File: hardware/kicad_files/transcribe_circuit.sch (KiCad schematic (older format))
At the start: 23 parts, among them J1 europower, J2 RS232_SERIAL, J3 RS232_DSUB, J4 MIDI_IN_TRS, J5 MIDI_IN_DIN, J6 MIDI_OUT_TRS, J7 MIDI_OUT_DIN, U1 ProMicro, U2 MAX232, U3 6N137, U4 4069, U5 usbHostMini, U6 L78L33_TO92

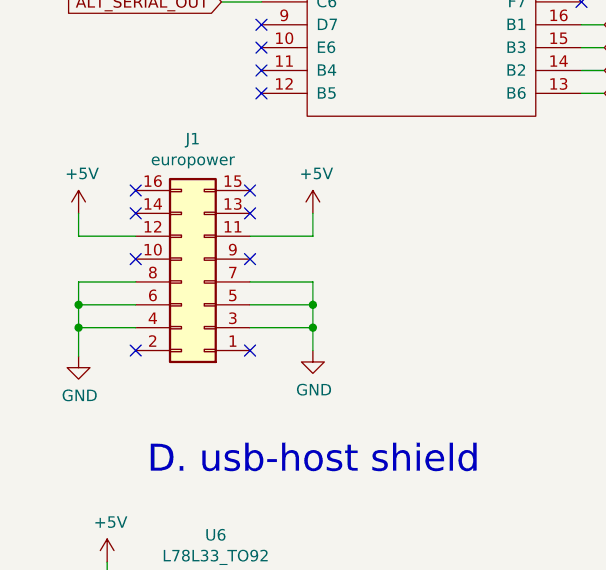
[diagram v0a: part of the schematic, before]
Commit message: small pcb fixes
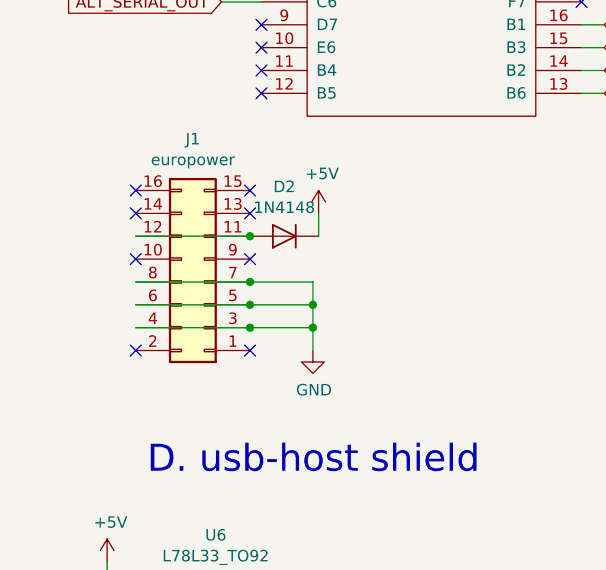
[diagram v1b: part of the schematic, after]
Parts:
- added D2: 1N4148, Diode_THT:D_T-1_P5.08mm_Horizontal, symbol Device:D
- C1: footprint Capacitor_THT:CP_Radial_D6.3mm_P2.50mm -> Capacitor_THT:CP_Radial_D5.0mm_P2.50mm
- C2, C3, C4, C5: footprint Capacitor_THT:C_Disc_D3.0mm_W1.6mm_P2.50mm -> Capacitor_THT:C_Disc_D4.3mm_W1.9mm_P5.00mm
- D1: footprint Diode_THT:D_A-405_P7.62mm_Horizontal -> Diode_THT:D_T-1_P5.08mm_Horizontal
- J1: footprint Connector_PinHeader_2.54mm:PinHeader_2x08_P2.54mm_Vertical -> lib_fp:PinHeader_2x08_P2.54_Euro
- J2, J4, J6: footprint Connector_Audio:Tayda_3.5mm_stereo_TRS_jack_A-853 -> lib_fp:Tayda_3.5mm_stereo_TRS_jack_A-853
- J5, J7: footprint Connector_DIN:Tayda5pinMidi-A1010 -> lib_fp:Tayda5pinMidi-A1010
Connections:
- net +5V: now also D2.1 (K); no longer J1.11 (Pin_11), J1.12 (Pin_12)
- new net: D2.2 (A), J1.11 (Pin_11), J1.12 (Pin_12)
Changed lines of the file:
@@
 F 0 "D1" V 8529 2129 50  0000 L CNN
 F 1 "1N4148" H 8475 1950 50  0000 L CNN
-F 2 "Diode_THT:D_A-405_P7.62mm_Horizontal" H 8575 2050 50  0001 C CNN
+F 2 "Diode_THT:D_T-1_P5.08mm_Horizontal" H 8575 2050 50  0001 C CNN
 F 3 "~" H 8575 2050 50  0001 C CNN
 	1    8575 2050
@@
 F 0 "J4" H 7632 3700 50  0000 C CNN
 F 1 "MIDI_IN_TRS" H 7632 3609 50  0000 C CNN
-F 2 "Connector_Audio:Tayda_3.5mm_stereo_TRS_jack_A-853" H 7650 3375 50  0001 C CNN
+F 2 "lib_fp:Tayda_3.5mm_stereo_TRS_jack_A-853" H 7650 3375 50  0001 C CNN
 F 3 "~" H 7650 3375 50  0001 C CNN
 	1    7650 3375
@@
 F 0 "J6" H 7707 6025 50  0000 C CNN
 F 1 "MIDI_OUT_TRS" H 7707 5934 50  0000 C CNN
-F 2 "Connector_Audio:Tayda_3.5mm_stereo_TRS_jack_A-853" H 7725 5700 50  0001 C CNN
+F 2 "lib_fp:Tayda_3.5mm_stereo_TRS_jack_A-853" H 7725 5700 50  0001 C CNN
 F 3 "~" H 7725 5700 50  0001 C CNN
 	1    7725 5700
@@
 F 0 "C2" H 4265 2971 50  0000 L CNN
 F 1 "0.1u" H 4265 2880 50  0000 L CNN
-F 2 "Capacitor_THT:C_Disc_D3.0mm_W1.6mm_P2.50mm" H 4188 2775 50  0001 C CNN
+F 2 "Capacitor_THT:C_Disc_D4.3mm_W1.9mm_P5.00mm" H 4188 2775 50  0001 C CNN
 F 3 "~" H 4150 2925 50  0001 C CNN
 	1    4150 2925
@@
 F 0 "C4" H 6365 2971 50  0000 L CNN
 F 1 "0.1u" H 6365 2880 50  0000 L CNN
-F 2 "Capacitor_THT:C_Disc_D3.0mm_W1.6mm_P2.50mm" H 6288 2775 50  0001 C CNN
+F 2 "Capacitor_THT:C_Disc_D4.3mm_W1.9mm_P5.00mm" H 6288 2775 50  0001 C CNN
 F 3 "~" H 6250 2925 50  0001 C CNN
 	1    6250 2925
@@
 F 0 "C3" V 6000 3275 50  0000 C CNN
 F 1 "0.1u" V 6300 3275 50  0000 C CNN
-F 2 "Capacitor_THT:C_Disc_D3.0mm_W1.6mm_P2.50mm" H 6188 3125 50  0001 C CNN
+F 2 "Capacitor_THT:C_Disc_D4.3mm_W1.9mm_P5.00mm" H 6188 3125 50  0001 C CNN
 F 3 "~" H 6150 3275 50  0001 C CNN
 	1    6150 3275
@@
 F 0 "C5" V 6150 3575 50  0000 C CNN
 F 1 "0.1u" V 6450 3575 50  0000 C CNN
-F 2 "Capacitor_THT:C_Disc_D3.0mm_W1.6mm_P2.50mm" H 6338 3425 50  0001 C CNN
+F 2 "Capacitor_THT:C_Disc_D4.3mm_W1.9mm_P5.00mm" H 6338 3425 50  0001 C CNN
 F 3 "~" H 6300 3575 50  0001 C CNN
 	1    6300 3575
@@
 F 0 "J2" H 4132 1900 50  0000 C CNN
 F 1 "RS232_SERIAL" H 4025 1800 50  0000 C CNN
-F 2 "Connector_Audio:Tayda_3.5mm_stereo_TRS_jack_A-853" H 4150 1575 50  0001 C CNN
+F 2 "lib_fp:Tayda_3.5mm_stereo_TRS_jack_A-853" H 4150 1575 50  0001 C CNN
 F 3 "~" H 4150 1575 50  0001 C CNN
 	1    4150 1575
@@
 F 0 "J7" H 9950 5525 50  0000 C CNN
 F 1 "MIDI_OUT_DIN" H 9950 5434 50  0000 C CNN
-F 2 "Connector_DIN:Tayda5pinMidi-A1010" H 9950 5800 50  0001 C CNN
+F 2 "lib_fp:Tayda5pinMidi-A1010" H 9950 5800 50  0001 C CNN
 F 3 "http://www.mouser.com/ds/2/18/40_c091_abd_e-75918.pdf" H 9950 5800 50  0001 C CNN
 	1    9950 5800
@@
 F 0 "J5" H 9850 3025 50  0000 C CNN
 F 1 "MIDI_IN_DIN" H 9850 2934 50  0000 C CNN
-F 2 "Connector_DIN:Tayda5pinMidi-A1010" H 9850 3300 50  0001 C CNN
+F 2 "lib_fp:Tayda5pinMidi-A1010" H 9850 3300 50  0001 C CNN
 F 3 "http://www.mouser.com/ds/2/18/40_c091_abd_e-75918.pdf" H 9850 3300 50  0001 C CNN
 	1    9850 3300
@@
 F 0 "C1" H 3618 1721 50  0000 L CNN
 F 1 "100uf" H 3618 1630 50  0000 L CNN
-F 2 "Capacitor_THT:CP_Radial_D6.3mm_P2.50mm" H 3538 1525 50  0001 C CNN
+F 2 "Capacitor_THT:CP_Radial_D5.0mm_P2.50mm" H 3538 1525 50  0001 C CNN
 F 3 "~" H 3500 1675 50  0001 C CNN
 	1    3500 1675
@@
 F 0 "J1" H 1300 3050 50  0000 C CNN
 F 1 "europower" H 1300 3141 50  0000 C CNN
-F 2 "Connector_PinHeader_2.54mm:PinHeader_2x08_P2.54mm_Vertical" H 1250 3675 50  0001 C CNN
+F 2 "lib_fp:PinHeader_2x08_P2.54_Euro" H 1250 3675 50  0001 C CNN
 F 3 "~" H 1250 3675 50  0001 C CNN
 	1    1250 3675
@@
 L power:+5V #PWR06
 U 1 1 5E281F93
-P 1725 3375
-F 0 "#PWR06" H 1725 3225 50  0001 C CNN
-F 1 "+5V" H 1740 3548 50  0000 C CNN
-F 2 "" H 1725 3375 50  0001 C CNN
-F 3 "" H 1725 3375 50  0001 C CNN
-	1    1725 3375
-	1    0    0    -1
-$EndComp
-$Comp
-L power:+5V #PWR01
-U 1 1 5E2863EC
-P 700 3375
-F 0 "#PWR01" H 700 3225 50  0001 C CNN
-F 1 "+5V" H 715 3548 50  0000 C CNN
-F 2 "" H 700 3375 50  0001 C CNN
-F 3 "" H 700 3375 50  0001 C CNN
-	1    700  3375
-	1    0    0    -1
-$EndComp
-Wire Wire Line
-	950  3475 700  3475
-Wire Wire Line
-	700  3475 700  3375
+P 1750 3375
+F 0 "#PWR06" H 1750 3225 50  0001 C CNN
+F 1 "+5V" H 1765 3548 50  0000 C CNN
+F 2 "" H 1750 3375 50  0001 C CNN
+F 3 "" H 1750 3375 50  0001 C CNN
+	1    1750 3375
+	1    0    0    -1
+$EndComp
 NoConn ~ 950  3275
 NoConn ~ 950  3375
@@
 NoConn ~ 1450 3575
 NoConn ~ 950  3575
-$Comp
-L power:GND #PWR02
-U 1 1 5E29F868
-P 700 4000
-F 0 "#PWR02" H 700 3750 50  0001 C CNN
-F 1 "GND" H 705 3827 50  0000 C CNN
-F 2 "" H 700 4000 50  0001 C CNN
-F 3 "" H 700 4000 50  0001 C CNN
-	1    700  4000
-	1    0    0    -1
-$EndComp
 $Comp
 L power:GND #PWR07
@@
 $EndComp
 Wire Wire Line
-	950  3675 700  3675
-Wire Wire Line
-	700  3675 700  3775
-Wire Wire Line
-	950  3875 700  3875
-Connection ~ 700  3875
-Wire Wire Line
-	700  3875 700  4000
-Wire Wire Line
-	950  3775 700  3775
-Connection ~ 700  3775
-Wire Wire Line
-	700  3775 700  3875
-Wire Wire Line
-	1725 3475 1725 3375
-Wire Wire Line
-	1450 3475 1725 3475
-Wire Wire Line
 	1450 3675 1725 3675
 Wire Wire Line
@@
 Wire Wire Line
 	6225 2050 6225 2125
+$Comp
+L Device:D D2
+U 1 1 5E8284AF
+P 1600 3475
+F 0 "D2" H 1600 3259 50  0000 C CNN
+F 1 "1N4148" H 1600 3350 50  0000 C CNN
+F 2 "Diode_THT:D_T-1_P5.08mm_Horizontal" H 1600 3475 50  0001 C CNN
+F 3 "~" H 1600 3475 50  0001 C CNN
+	1    1600 3475
+	-1   0    0    1
+$EndComp
+Wire Wire Line
+	1750 3375 1750 3475
+Wire Wire Line
+	950  3475 1450 3475
+Connection ~ 1450 3475
+Wire Wire Line
+	950  3675 1450 3675
+Connection ~ 1450 3675
+Wire Wire Line
+	950  3775 1450 3775
+Connection ~ 1450 3775
+Wire Wire Line
+	950  3875 1450 3875
+Connection ~ 1450 3875
 $EndSCHEMATC
